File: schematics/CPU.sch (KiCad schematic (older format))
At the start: 6 parts

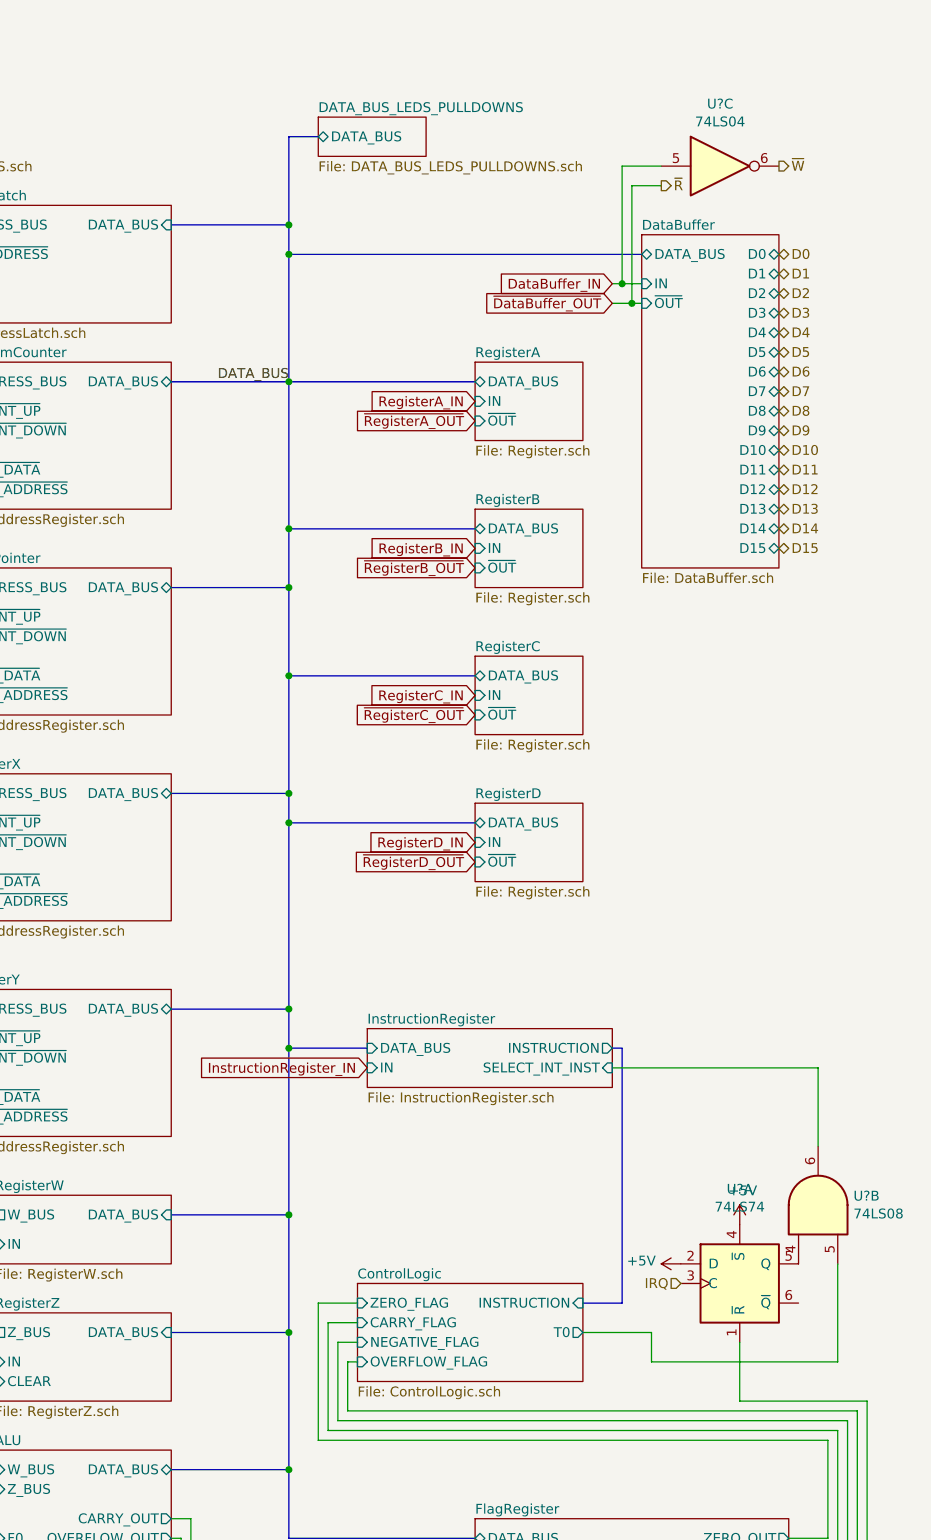
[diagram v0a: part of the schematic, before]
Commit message: update schematics
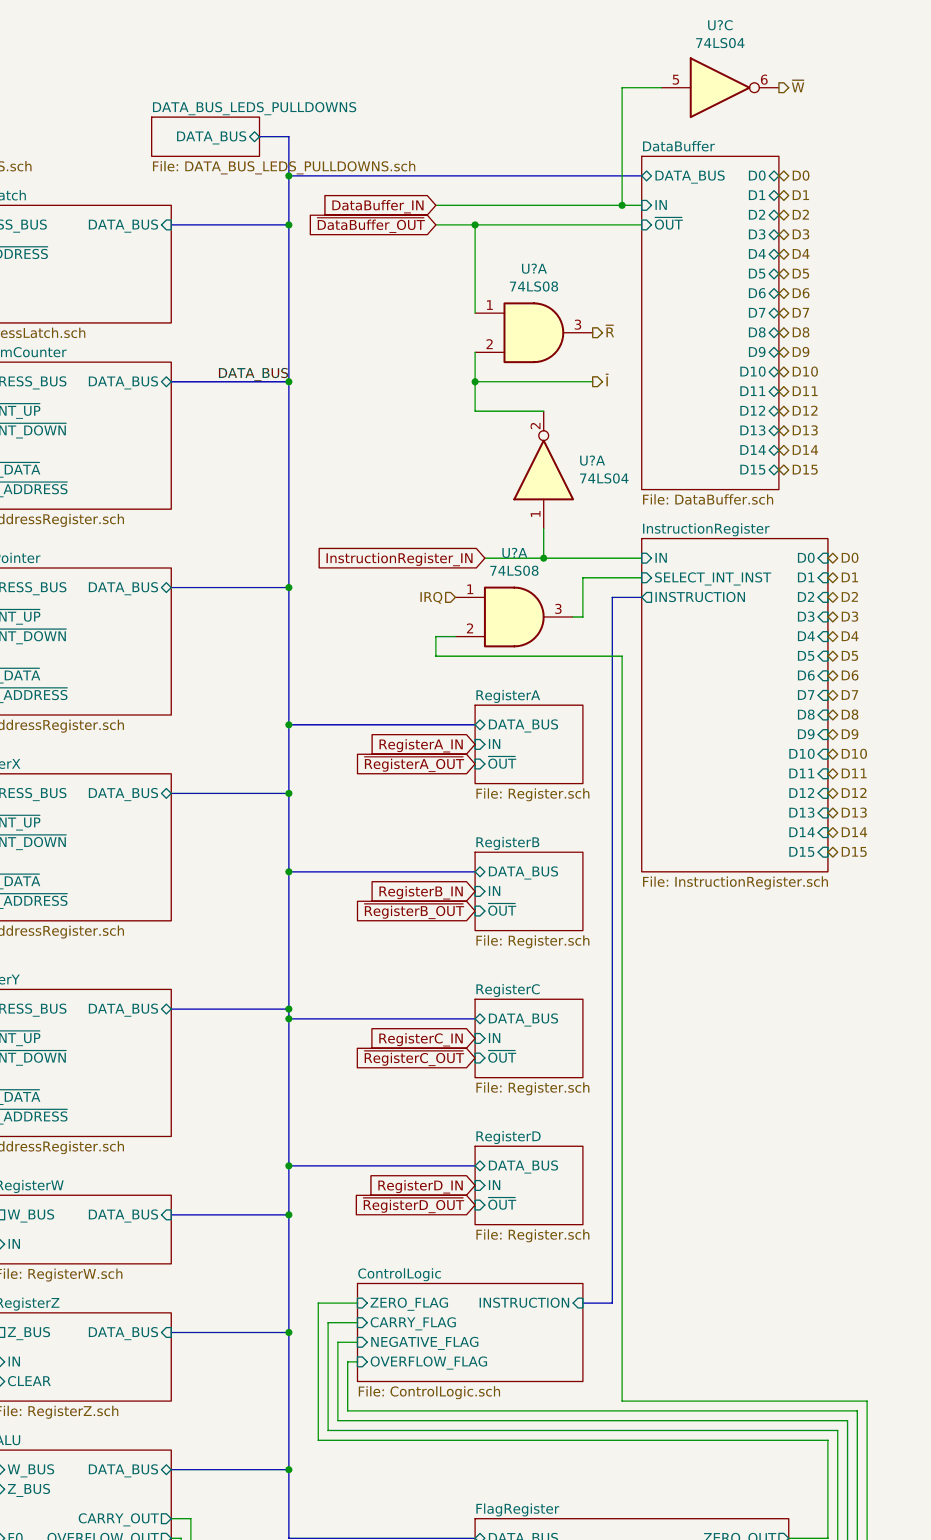
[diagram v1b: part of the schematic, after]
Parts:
- removed U?: 74LS74, symbol 74xx:74LS74
- removed U?: 74LS08, symbol 74xx:74LS08
- added U?: 74LS04, symbol 74xx:74LS04
- added U? (x2): 74LS08, symbol 74xx:74LS08
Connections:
- net FlagRegister/INTERRUPT_ENABLE_OUT: now also U?.2
- net IRQ: now also U?.1
- net InstructionRegister/SELECT_INT_INST: now also U?.3
- net InstructionRegister_IN: now also U?.1
- net ~DataBuffer_OUT: now also U?.1
- new net ~I: U?.2, U?.2
- new net ~R: U?.3
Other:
- moved on the sheet: U?C

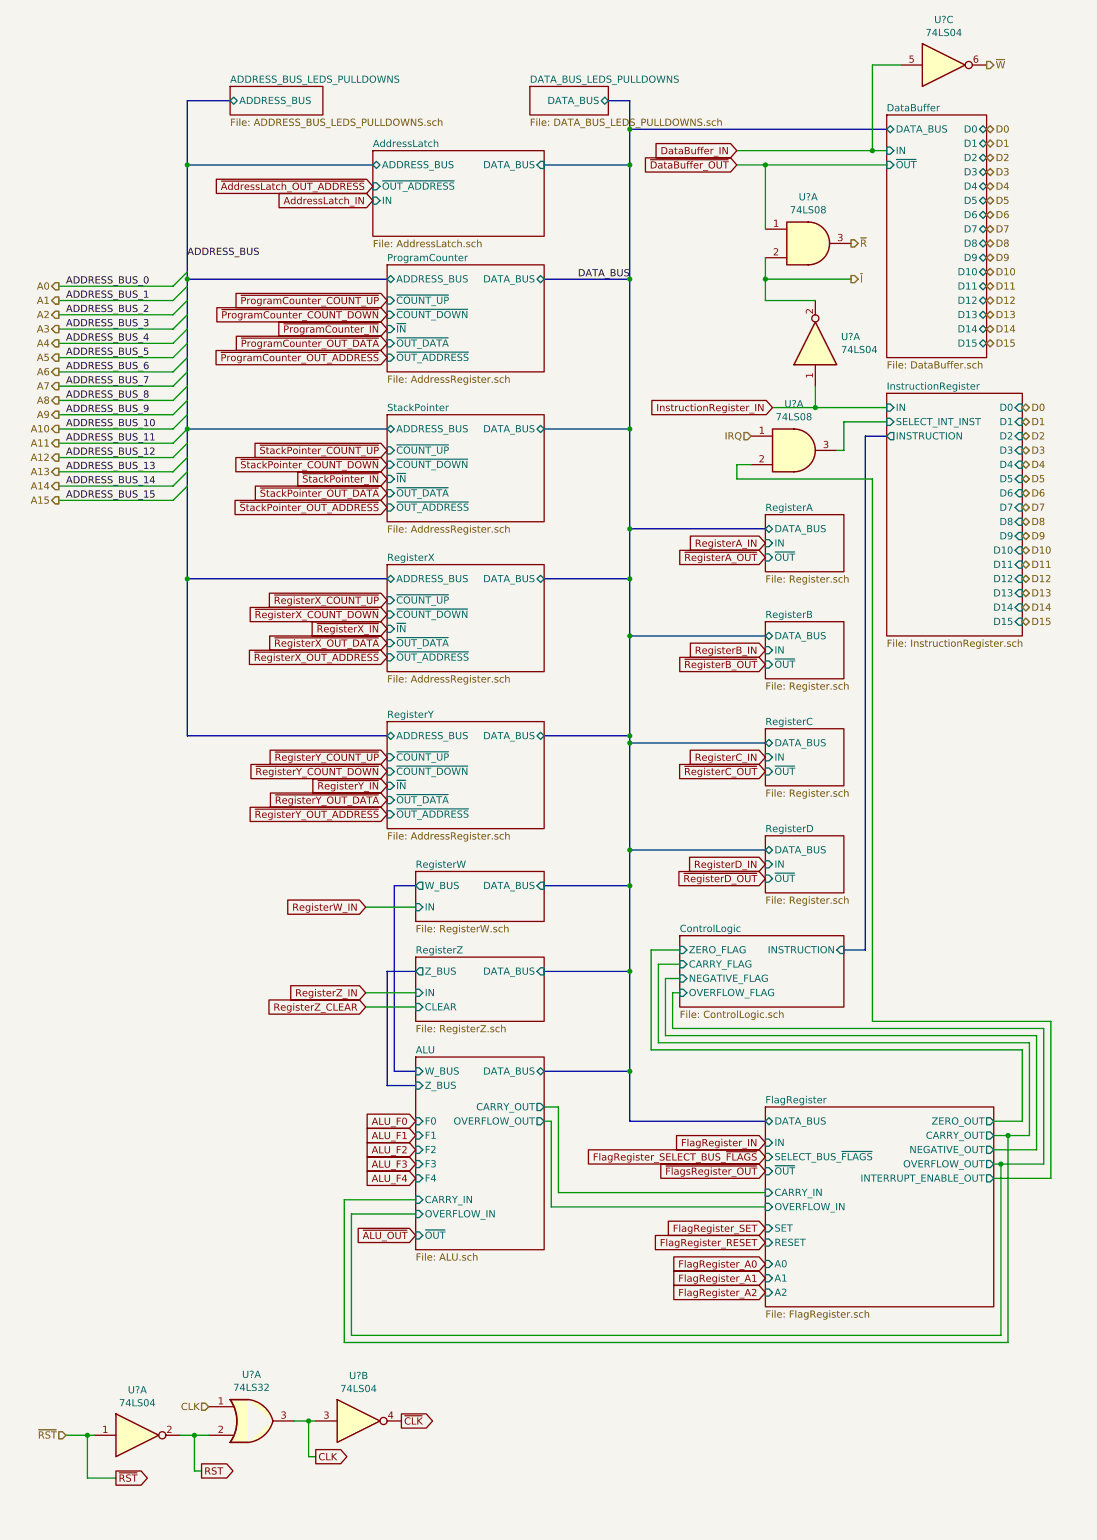
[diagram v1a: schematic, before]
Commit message: update schematics
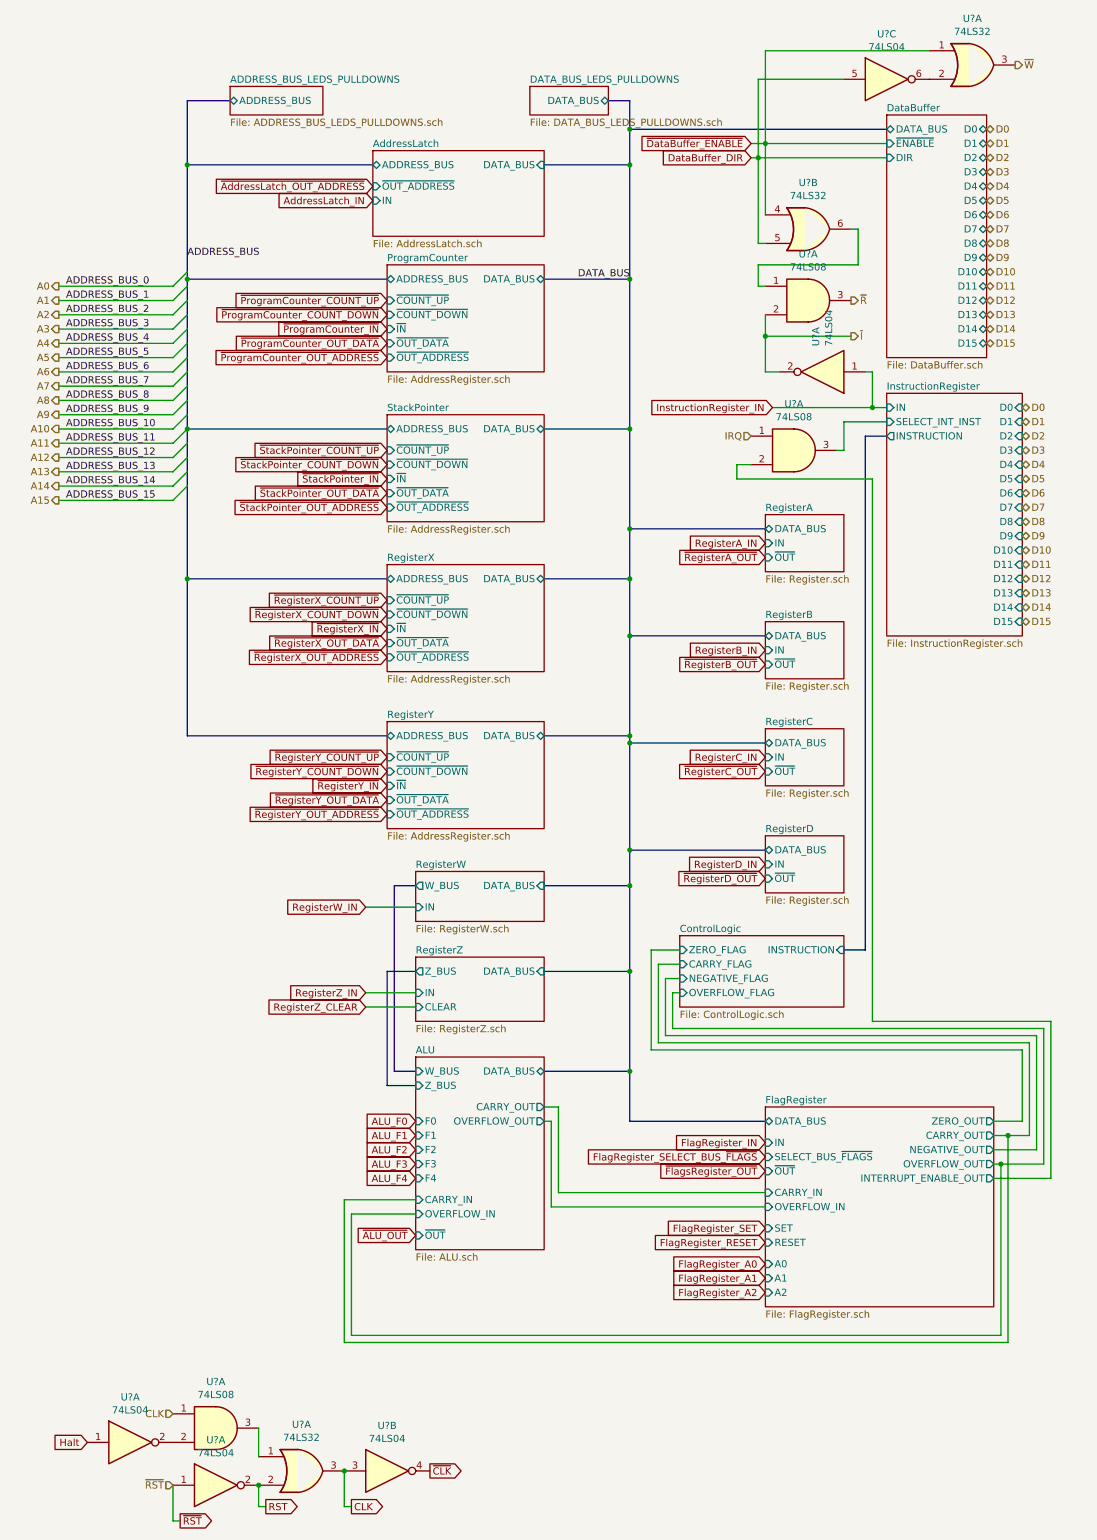
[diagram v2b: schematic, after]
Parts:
- added U? (x2): 74LS32, symbol 74xx:74LS32
- added U?: 74LS08, symbol 74xx:74LS08
- added U?: 74LS04, symbol 74xx:74LS04
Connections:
- net CLK: now also U?.1; no longer U?.1
- net ~W: now also U?.3; no longer U?.6
- net DataBuffer_IN renamed DataBuffer_DIR
- net DataBuffer_DIR: now also U?.5
- net ~DataBuffer_OUT: no longer names the net of U?.1
- net ~DataBuffer_OUT: now also U?.6
- new net: U?.1, U?.3
- new net: U?.2, U?.6
- new net: U?.2, U?.2
- new net Halt: U?.1
- new net ~DataBuffer_ENABLE: U?.1, U?.4
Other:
- moved on the sheet: U?A, U?B, U?C
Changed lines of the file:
@@
 F17 "D14" T R 7200 2700 50
 F18 "D15" T R 7200 2800 50
-F19 "IN" I L 6500 1450 50
-F20 "~OUT" I L 6500 1550 50
+F19 "~ENABLE" I L 6500 1400 50
+F20 "DIR" I L 6500 1500 50
 $EndSheet
 Wire Bus Line
@@
 Text HLabel 7200 2800 2    50   3State ~ 0
 D15
-Text GLabel 5450 1450 0    50   Input ~ 0
-DataBuffer_IN
-Text GLabel 5450 1550 0    50   Input ~ 0
-~DataBuffer_OUT
 Wire Bus Line
 	4700 1300 6500 1300
@@
 Wire Bus Line
 	4100 1550 4700 1550
-Text HLabel 7200 850  2    50   Output ~ 0
+Text HLabel 7400 850  2    50   Output ~ 0
 ~W
-Text HLabel 6250 2100 2    50   Output ~ 0
+Text HLabel 6250 2500 2    50   Output ~ 0
 ~R
-Wire Wire Line
-	6400 1450 6400 850
-Wire Wire Line
-	6400 850  6600 850
-Connection ~ 6400 1450
-Wire Wire Line
-	6400 1450 6500 1450
 Wire Wire Line
 	5050 7350 5000 7350
@@
 Wire Wire Line
 	7450 8250 7250 8250
-Text HLabel 750  10450 0    50   Input ~ 0
+Text HLabel 1500 10800 0    50   Input ~ 0
 ~RST
-Text GLabel 1100 10750 2    50   Output ~ 0
+Text GLabel 1550 11050 2    50   Output ~ 0
 ~RST
 $Comp
 L 74xx:74LS04 U?
 U 1 1 5F1CEB9C
-P 1250 10450
-F 0 "U?" H 1250 10767 50  0000 C CNN
-F 1 "74LS04" H 1250 10676 50  0000 C CNN
-F 2 "" H 1250 10450 50  0001 C CNN
-F 3 "http://www.ti.com/lit/gpn/sn74LS04" H 1250 10450 50  0001 C CNN
-	1    1250 10450
+P 1800 10800
+F 0 "U?" H 1800 11117 50  0000 C CNN
+F 1 "74LS04" H 1800 11026 50  0000 C CNN
+F 2 "" H 1800 10800 50  0001 C CNN
+F 3 "http://www.ti.com/lit/gpn/sn74LS04" H 1800 10800 50  0001 C CNN
+	1    1800 10800
 	1    0    0    -1
 $EndComp
@@
 L 74xx:74LS32 U?
 U 1 1 5F1D28C6
-P 2050 10350
-F 0 "U?" H 2050 10675 50  0000 C CNN
-F 1 "74LS32" H 2050 10584 50  0000 C CNN
-F 2 "" H 2050 10350 50  0001 C CNN
-F 3 "http://www.ti.com/lit/gpn/sn74LS32" H 2050 10350 50  0001 C CNN
-	1    2050 10350
-	1    0    0    -1
-$EndComp
-Text HLabel 1750 10250 0    50   Input ~ 0
+P 2400 10700
+F 0 "U?" H 2400 11025 50  0000 C CNN
+F 1 "74LS32" H 2400 10934 50  0000 C CNN
+F 2 "" H 2400 10700 50  0001 C CNN
+F 3 "http://www.ti.com/lit/gpn/sn74LS32" H 2400 10700 50  0001 C CNN
+	1    2400 10700
+	1    0    0    -1
+$EndComp
+Text HLabel 1500 10300 0    50   Input ~ 0
 CLK
-Wire Wire Line
-	1550 10450 1650 10450
-Wire Wire Line
-	750  10450 900  10450
-Wire Wire Line
-	900  10450 900  10750
-Wire Wire Line
-	900  10750 1100 10750
-Connection ~ 900  10450
-Wire Wire Line
-	900  10450 950  10450
 $Comp
 L 74xx:74LS04 U?
 U 2 1 5F1EACAD
-P 2800 10350
-F 0 "U?" H 2800 10667 50  0000 C CNN
-F 1 "74LS04" H 2800 10576 50  0000 C CNN
-F 2 "" H 2800 10350 50  0001 C CNN
-F 3 "http://www.ti.com/lit/gpn/sn74LS04" H 2800 10350 50  0001 C CNN
-	2    2800 10350
-	1    0    0    -1
-$EndComp
-Text GLabel 3100 10350 2    50   Output ~ 0
+P 3000 10700
+F 0 "U?" H 3000 11017 50  0000 C CNN
+F 1 "74LS04" H 3000 10926 50  0000 C CNN
+F 2 "" H 3000 10700 50  0001 C CNN
+F 3 "http://www.ti.com/lit/gpn/sn74LS04" H 3000 10700 50  0001 C CNN
+	2    3000 10700
+	1    0    0    -1
+$EndComp
+Text GLabel 3300 10700 2    50   Output ~ 0
 ~CLK
-Text GLabel 2500 10600 2    50   Output ~ 0
+Text GLabel 2750 10950 2    50   Output ~ 0
 CLK
-Wire Wire Line
-	2350 10350 2450 10350
-Wire Wire Line
-	2500 10600 2450 10600
-Wire Wire Line
-	2450 10600 2450 10350
-Connection ~ 2450 10350
-Wire Wire Line
-	2450 10350 2500 10350
 $Comp
 L 74xx:74LS04 U?
 U 3 1 5F2108AC
-P 6900 850
-F 0 "U?" H 6900 1167 50  0000 C CNN
-F 1 "74LS04" H 6900 1076 50  0000 C CNN
-F 2 "" H 6900 850 50  0001 C CNN
-F 3 "http://www.ti.com/lit/gpn/sn74LS04" H 6900 850 50  0001 C CNN
-	3    6900 850
+P 6500 950
+F 0 "U?" H 6500 1267 50  0000 C CNN
+F 1 "74LS04" H 6500 1176 50  0000 C CNN
+F 2 "" H 6500 950 50  0001 C CNN
+F 3 "http://www.ti.com/lit/gpn/sn74LS04" H 6500 950 50  0001 C CNN
+	3    6500 950
 	1    0    0    -1
 $EndComp
@@
 F8 "~COUNT_UP" I L 3000 2500 50
 $EndSheet
-Text GLabel 1700 10700 2    50   Output ~ 0
+Text GLabel 2150 10950 2    50   Output ~ 0
 RST
-Wire Wire Line
-	1700 10700 1650 10700
-Wire Wire Line
-	1650 10700 1650 10450
-Connection ~ 1650 10450
-Wire Wire Line
-	1650 10450 1750 10450
 Wire Bus Line
 	4700 5550 4700 5600
@@
 L 74xx:74LS04 U?
 U 1 1 612083D0
-P 6000 2800
-F 0 "U?" V 6046 2620 50  0000 R CNN
-F 1 "74LS04" V 5955 2620 50  0000 R CNN
-F 2 "" H 6000 2800 50  0001 C CNN
-F 3 "http://www.ti.com/lit/gpn/sn74LS04" H 6000 2800 50  0001 C CNN
-	1    6000 2800
-	0    -1   -1   0
-$EndComp
-Wire Wire Line
-	5700 3250 6000 3250
-Wire Wire Line
-	6000 3100 6000 3250
-Connection ~ 6000 3250
-Wire Wire Line
-	6000 3250 6500 3250
+P 6050 3000
+F 0 "U?" V 6096 2820 50  0000 R CNN
+F 1 "74LS04" V 6005 2820 50  0000 R CNN
+F 2 "" H 6050 3000 50  0001 C CNN
+F 3 "http://www.ti.com/lit/gpn/sn74LS04" H 6050 3000 50  0001 C CNN
+	1    6050 3000
+	-1   0    0    1
+$EndComp
 $Comp
 L 74xx:74LS08 U?
 U 1 1 6121832D
-P 5950 2100
-F 0 "U?" H 5950 2425 50  0000 C CNN
-F 1 "74LS08" H 5950 2334 50  0000 C CNN
-F 2 "" H 5950 2100 50  0001 C CNN
-F 3 "http://www.ti.com/lit/gpn/sn74LS08" H 5950 2100 50  0001 C CNN
-	1    5950 2100
-	1    0    0    -1
-$EndComp
-Wire Wire Line
-	6000 2500 5650 2500
-Wire Wire Line
-	5650 2500 5650 2350
-Wire Wire Line
-	5450 1550 5650 1550
-Wire Wire Line
-	5650 2000 5650 1550
-Connection ~ 5650 1550
-Wire Wire Line
-	5650 1550 6500 1550
-Wire Wire Line
-	5450 1450 6400 1450
-Text HLabel 6250 2350 2    50   Output ~ 0
+P 5950 2500
+F 0 "U?" H 5950 2825 50  0000 C CNN
+F 1 "74LS08" H 5950 2734 50  0000 C CNN
+F 2 "" H 5950 2500 50  0001 C CNN
+F 3 "http://www.ti.com/lit/gpn/sn74LS08" H 5950 2500 50  0001 C CNN
+	1    5950 2500
+	1    0    0    -1
+$EndComp
+Text HLabel 6250 2750 2    50   Output ~ 0
 ~I
 Wire Wire Line
-	6250 2350 5650 2350
-Connection ~ 5650 2350
-Wire Wire Line
-	5650 2350 5650 2200
+	6250 2750 5650 2750
 $Comp
 L 74xx:74LS08 U?
@@
 	6350 3450 6350 7050
 Wire Bus Line
+	6200 7050 6350 7050
+$Comp
+L 74xx:74LS08 U?
+U 1 1 6093B661
+P 1800 10400
+F 0 "U?" H 1800 10725 50  0000 C CNN
+F 1 "74LS08" H 1800 10634 50  0000 C CNN
+F 2 "" H 1800 10400 50  0001 C CNN
+F 3 "http://www.ti.com/lit/gpn/sn74LS08" H 1800 10400 50  0001 C CNN
+	1    1800 10400
+	1    0    0    -1
+$EndComp
+$Comp
+L 74xx:74LS04 U?
+U 1 1 6094548C
+P 1200 10500
+F 0 "U?" H 1200 10817 50  0000 C CNN
+F 1 "74LS04" H 1200 10726 50  0000 C CNN
+F 2 "" H 1200 10500 50  0001 C CNN
+F 3 "http://www.ti.com/lit/gpn/sn74LS04" H 1200 10500 50  0001 C CNN
+	1    1200 10500
+	1    0    0    -1
+$EndComp
+Text GLabel 900  10500 0    50   Input ~ 0
+Halt
+Wire Wire Line
+	2700 10700 2700 10950
+Connection ~ 2700 10700
+Wire Wire Line
+	2700 10950 2750 10950
+Wire Wire Line
+	2100 10800 2100 10950
+Wire Wire Line
+	2100 10950 2150 10950
+Connection ~ 2100 10800
+Wire Wire Line
+	1500 10800 1500 11050
+Wire Wire Line
+	1500 11050 1550 11050
+Wire Wire Line
+	2100 10400 2100 10600
+$Comp
+L 74xx:74LS32 U?
+U 1 1 607CCE4C
+P 7100 850
+F 0 "U?" H 7100 1175 50  0000 C CNN
+F 1 "74LS32" H 7100 1084 50  0000 C CNN
+F 2 "" H 7100 850 50  0001 C CNN
+F 3 "http://www.ti.com/lit/gpn/sn74LS32" H 7100 850 50  0001 C CNN
+	1    7100 850
+	1    0    0    -1
+$EndComp
+$Comp
+L 74xx:74LS32 U?
+U 2 1 607FCF88
+P 5950 2000
+F 0 "U?" H 5950 2325 50  0000 C CNN
+F 1 "74LS32" H 5950 2234 50  0000 C CNN
+F 2 "" H 5950 2000 50  0001 C CNN
+F 3 "http://www.ti.com/lit/gpn/sn74LS32" H 5950 2000 50  0001 C CNN
+	2    5950 2000
+	1    0    0    -1
+$EndComp
+Text GLabel 5550 1400 0    50   Input ~ 0
+~DataBuffer_ENABLE
+Text GLabel 5550 1500 0    50   Input ~ 0
+DataBuffer_DIR
+Wire Wire Line
+	5700 3250 6400 3250
+Wire Wire Line
+	6350 3000 6400 3000
+Wire Wire Line
+	6400 3000 6400 3250
+Connection ~ 6400 3250
+Wire Wire Line
+	6400 3250 6500 3250
+Wire Wire Line
+	5750 3000 5650 3000
+Wire Wire Line
+	5650 3000 5650 2750
+Wire Wire Line
+	5650 2600 5650 2750
+Connection ~ 5650 2750
+Wire Wire Line
+	6250 2000 6300 2000
+Wire Wire Line
+	6300 2000 6300 2250
+Wire Wire Line
+	6300 2250 5600 2250
+Wire Wire Line
+	5600 2250 5600 2400
+Wire Wire Line
+	5600 2400 5650 2400
+Wire Wire Line
+	5550 1400 5650 1400
+Wire Wire Line
+	5550 1500 5600 1500
+Wire Wire Line
+	5600 2100 5650 2100
+Connection ~ 5650 1400
+Wire Wire Line
+	5650 1400 5650 750
+Wire Wire Line
+	5650 750  6800 750
+Wire Wire Line
+	5650 1400 6500 1400
+Wire Wire Line
+	5650 1400 5650 1900
+Wire Wire Line
+	5600 1500 5600 2100
+Wire Wire Line
+	5600 1500 5600 950
+Wire Wire Line
+	5600 950  6200 950
+Connection ~ 5600 1500
+Wire Wire Line
+	5600 1500 6500 1500
+Wire Bus Line
 	1600 1550 1600 2350
 Wire Bus Line
-	6200 7050 6350 7050
-Wire Bus Line
 	1600 3400 1600 4450
